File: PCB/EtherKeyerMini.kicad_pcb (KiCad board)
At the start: 2 copper layers, 70 x 50 mm, 32 parts, among them J1 Key Output, J2 Paddle Input, J3 UART, Q2 2N4401, Q3 2N4401, SW1 Power Switch, U1 ATtiny85

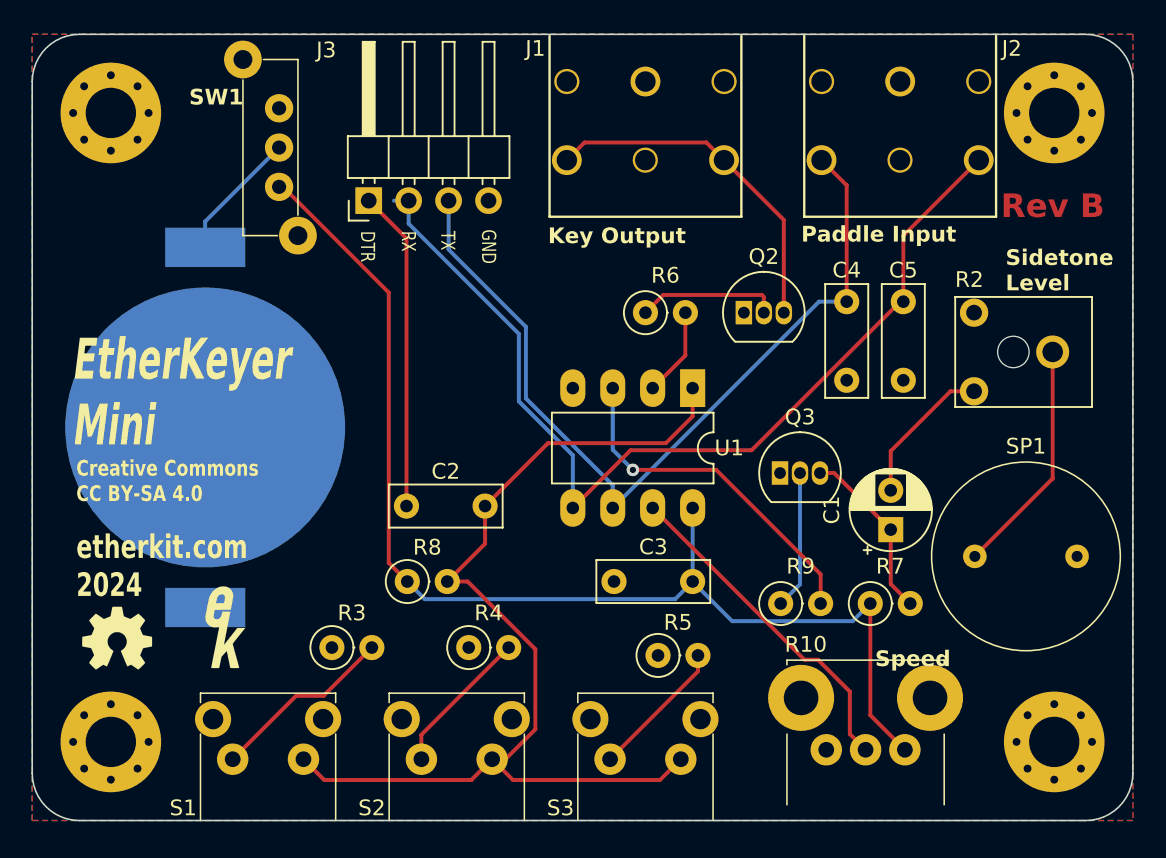
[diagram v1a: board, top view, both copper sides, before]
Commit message: Rev C PCB
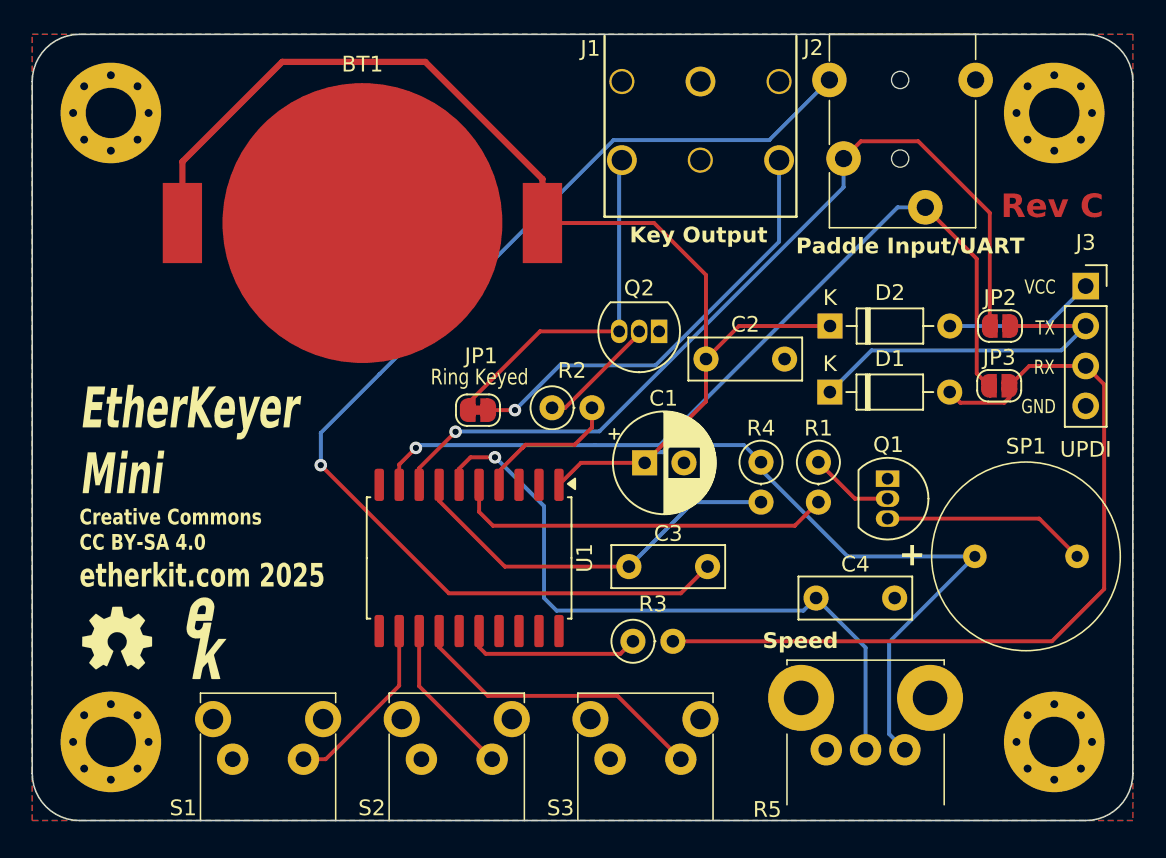
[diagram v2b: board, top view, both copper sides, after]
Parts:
- removed C5: 100n, Capacitor_THT:C_Rect_L7.0mm_W2.5mm_P5.00mm
- removed Q3: 2N4401, Package_TO_SOT_THT:TO-92_Inline
- removed R10: 1M, EtherkitKicadLibrary:Bournes_PTV09A
- removed R6, R8, R9: 10k, Resistor_THT:R_Axial_DIN0207_L6.3mm_D2.5mm_P2.54mm_Vertical
- removed R7: 3.3k, Resistor_THT:R_Axial_DIN0207_L6.3mm_D2.5mm_P2.54mm_Vertical
- removed SW1: Power Switch, EtherkitKicadLibrary:E-Switch_LC1258
- added D1: 1N5711, Diode_THT:D_DO-35_SOD27_P7.62mm_Horizontal, F.Cu at (150.7, 72.8)
- added D2: 1N5711, Diode_THT:D_DO-35_SOD27_P7.62mm_Horizontal, F.Cu at (150.7, 68.5)
- added JP1: Ring Keyed, Jumper:SolderJumper-2_P1.3mm_Bridged_RoundedPad1.0x1.5mm, F.Cu at (128.3, 73.9)
- added JP2: SolderJumper_2_Bridged, Jumper:SolderJumper-2_P1.3mm_Open_RoundedPad1.0x1.5mm, F.Cu at (161.6, 68.5)
- added JP3: SolderJumper_2_Bridged, Jumper:SolderJumper-2_P1.3mm_Open_RoundedPad1.0x1.5mm, F.Cu at (161.5, 72.3)
- added Q1: 2N4401, Package_TO_SOT_THT:TO-92_Inline, F.Cu at (154.4, 78.3)
- added R1: 10k, Resistor_THT:R_Axial_DIN0207_L6.3mm_D2.5mm_P2.54mm_Vertical, F.Cu at (150.0, 77.2)
- BT1: moved to F.Cu
- C1: value 10u -> 4.7u; footprint Capacitor_THT:CP_Radial_D5.0mm_P2.50mm -> Capacitor_THT:CP_Radial_D6.3mm_P2.50mm
- J2: value Paddle Input -> Paddle Input/UART; footprint EtherkitKicadLibrary:Kycon_STX-3120-3B -> EtherkitKicadLibrary:SameSky_SJ-43514
- J3: value UART -> UPDI; footprint Connector_PinHeader_2.54mm:PinHeader_1x04_P2.54mm_Horizontal -> Connector_PinSocket_2.54mm:PinSocket_1x04_P2.54mm_Vertical
- R2: footprint EtherkitKicadLibrary:Piher_N6L50T0C-103 -> Resistor_THT:R_Axial_DIN0207_L6.3mm_D2.5mm_P2.54mm_Vertical
- R3: value 10k -> 470
- R4: value 22k -> 10k
- R5: value 47k -> 1M; footprint Resistor_THT:R_Axial_DIN0207_L6.3mm_D2.5mm_P2.54mm_Vertical -> EtherkitKicadLibrary:Bournes_PTV09A
- SP1: value Speaker -> Piezo Speaker
- U1: value ATtiny85 -> ATtiny3226-S; footprint Package_DIP:DIP-8_W7.62mm_LongPads -> Package_SO:SOIC-20W_7.5x12.8mm_P1.27mm
- moved J3 45.9 mm to (167.0, 66.0), turned to 0 degrees
- moved R2 29.6 mm to (133.1, 73.8), turned to 0 degrees
- moved R4 22.0 mm to (146.3, 77.2), turned to -90 degrees
- moved C2 21.2 mm to (147.8, 70.7)
- moved R3 19.1 mm to (138.2, 88.6)
- moved C4 19.0 mm to (149.8, 85.8), turned to 0 degrees
- moved U1 17.9 mm to (127.8, 83.3)
- moved BT1 16.4 mm to (121.0, 62.0), turned to 0 degrees
- moved R5 16.3 mm to (153.0, 99.0)
- moved C1 16.2 mm to (138.9, 77.2), turned to 0 degrees
- moved Q2 5.52 mm to (139.9, 68.9), turned to 180 degrees
- moved C3 4.16 mm to (137.9, 83.8), turned to 0 degrees
- moved J1 3.50 mm to (142.5, 50.0)
- moved G1 1.39 mm to (111.1, 88.4)
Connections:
- BT1 pad 1: Net-(BT1-+) -> VDD
- C1 pad 1: Net-(Q3-C) -> VDD
- C1 pad 2: Net-(C1-Pad2) -> GND
- C2 pad 1: Net-(U1-PB5/RESET) -> GND
- C2 pad 2: DTR -> VDD
- C3 pad 1: VDD -> Net-(U1-PB4)
- C3 pad 2: GND -> DTR
- C4 pad 1: TX -> Net-(U1-PB5)
- J1 pad R: Net-(Q2-C) -> Net-(JP1-A)
- J1 pad T: Net-(Q2-C) -> Net-(JP1-B)
- J2 pad S: GND -> DTR
- J3 pad 1: DTR -> Net-(D2-A)
- J3 pad 2: RX -> Net-(D1-K)
- J3 pad 3: TX -> Net-(D1-A)
- Q2 pad 3: Net-(Q2-C) -> Net-(JP1-B)
- R2 pad 1: Net-(C1-Pad2) -> Net-(Q2-B)
- R2 pad 2: Net-(R2-Pad2) -> KEY
- R3 pad 1: GND -> Net-(U1-~{RESET}/PA0)
- R3 pad 2: Net-(R3-Pad2) -> Net-(D1-A)
- R4 pad 1: GND -> VDD
- R4 pad 2: Net-(R4-Pad2) -> Net-(U1-PB4)
- R5 pad 1: GND -> VDD
- R5 pad 2: Net-(R5-Pad2) -> Net-(U1-PB5)
- S1 pad 1: Net-(R3-Pad2) -> GND
- S1 pad 2: Net-(U1-PB5/RESET) -> Net-(U1-PC0)
- S2 pad 1: Net-(R4-Pad2) -> GND
- S2 pad 2: Net-(U1-PB5/RESET) -> Net-(U1-PC1)
- S3 pad 1: Net-(R5-Pad2) -> GND
- S3 pad 2: Net-(U1-PB5/RESET) -> Net-(U1-PC2)
- SP1 pad 1: Net-(R2-Pad2) -> VDD
- SP1 pad 2: GND -> Net-(Q1-C)
- U1 pad 1: Net-(U1-PB5/RESET) -> VDD
- U1 pad 2: Net-(U1-PB3) -> unconnected-(U1-PA4-Pad2)
- U1 pad 3: Net-(U1-PB4) -> unconnected-(U1-PA5-Pad3)
- U1 pad 4: GND -> KEY
- U1 pad 5: RX -> SIDETONE
- U1 pad 6: TX -> Net-(U1-PB5)
- U1 pad 7: Net-(U1-PB2) -> Net-(U1-PB4)
- U1 pad 8: VDD -> TX
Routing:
- net Net-(U1-PB5/RESET): track 65.4 -> 0.00 mm
- net Net-(D1-A): track 0.00 -> 53.8 mm
- net DTR: track 20.4 -> 72.4 mm, vias 0 -> 1
- net Net-(U1-PB5): track 0.00 -> 42.8 mm, vias 0 -> 1
- net VDD: track 75.4 -> 115.1 mm
- net Net-(JP1-A): track 0.00 -> 28.1 mm, vias 0 -> 1
- net SIDETONE: track 0.00 -> 24.3 mm
- net Net-(JP1-B): track 0.00 -> 22.9 mm
- net Net-(D1-K): track 0.00 -> 22.8 mm
- net Net-(Q2-C): track 22.2 -> 0.00 mm
- net Net-(U1-PB2): track 21.5 -> 0.00 mm
- net Net-(U1-PC2): track 0.00 -> 19.3 mm
- net Net-(R2-Pad2): track 15.1 -> 0.00 mm
- net Net-(Q1-C): track 0.00 -> 13.0 mm
- net Net-(R3-Pad2): track 11.8 -> 0.00 mm
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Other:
- board text added: "+"
- board text added: "Paddle Input/UART"
- board text added: "Rev C"
- board text added: "VCC"
- board text added: "etherkit.com 2025"
- board text removed: "DTR"
- board text removed: "Paddle Input"
- board text removed: "Rev B"
- board text removed: "Sidetone Level"
- board text removed: "etherkit.com 2024"
